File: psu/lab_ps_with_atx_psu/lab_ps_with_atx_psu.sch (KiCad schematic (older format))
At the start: 4 parts, among them CON1 +5V StandBy, U1 LD1117-33

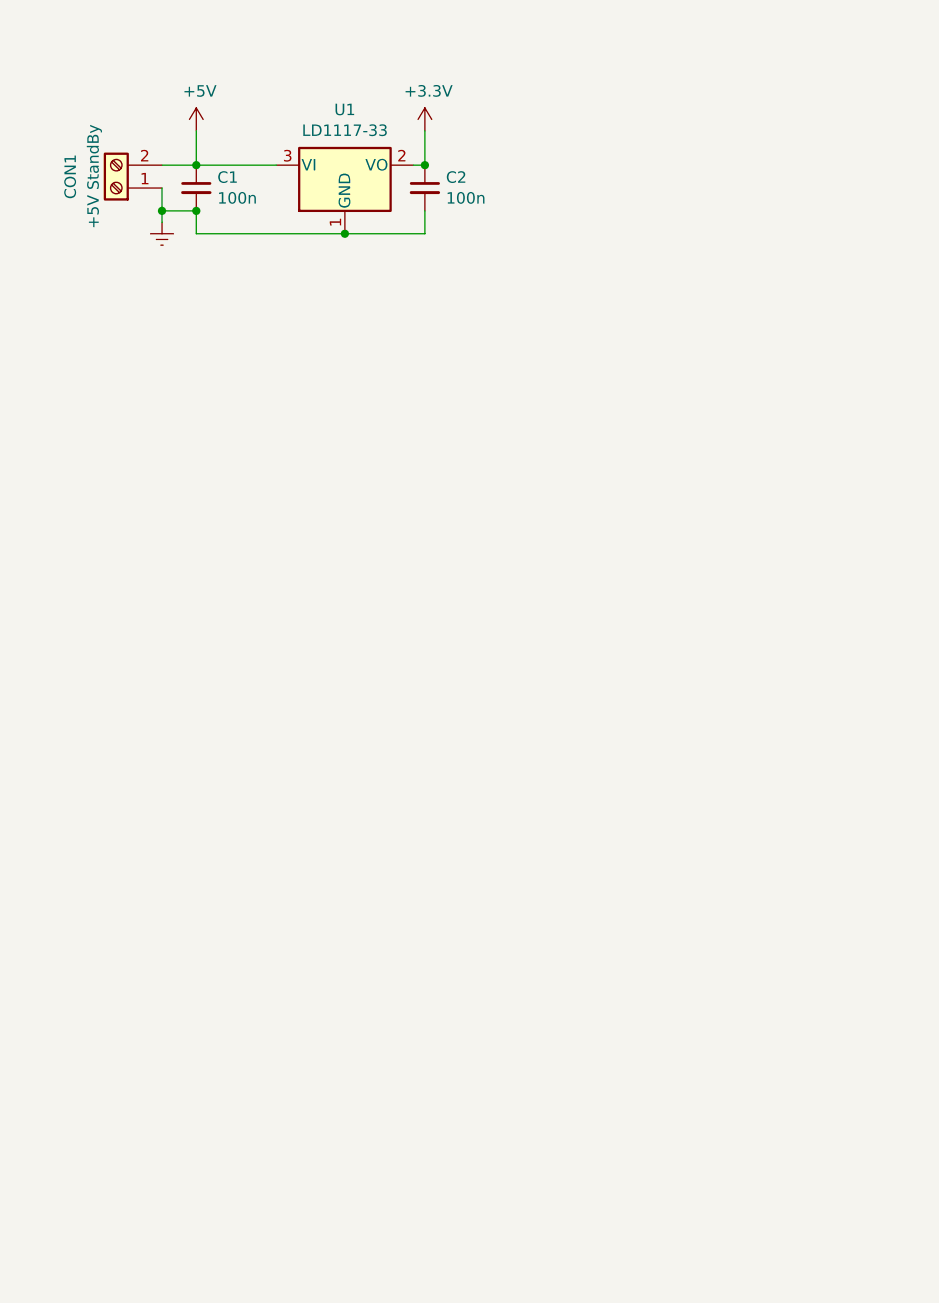
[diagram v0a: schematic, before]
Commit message: microcontroller is added
Please enter the commit message for your changes. Lines starting
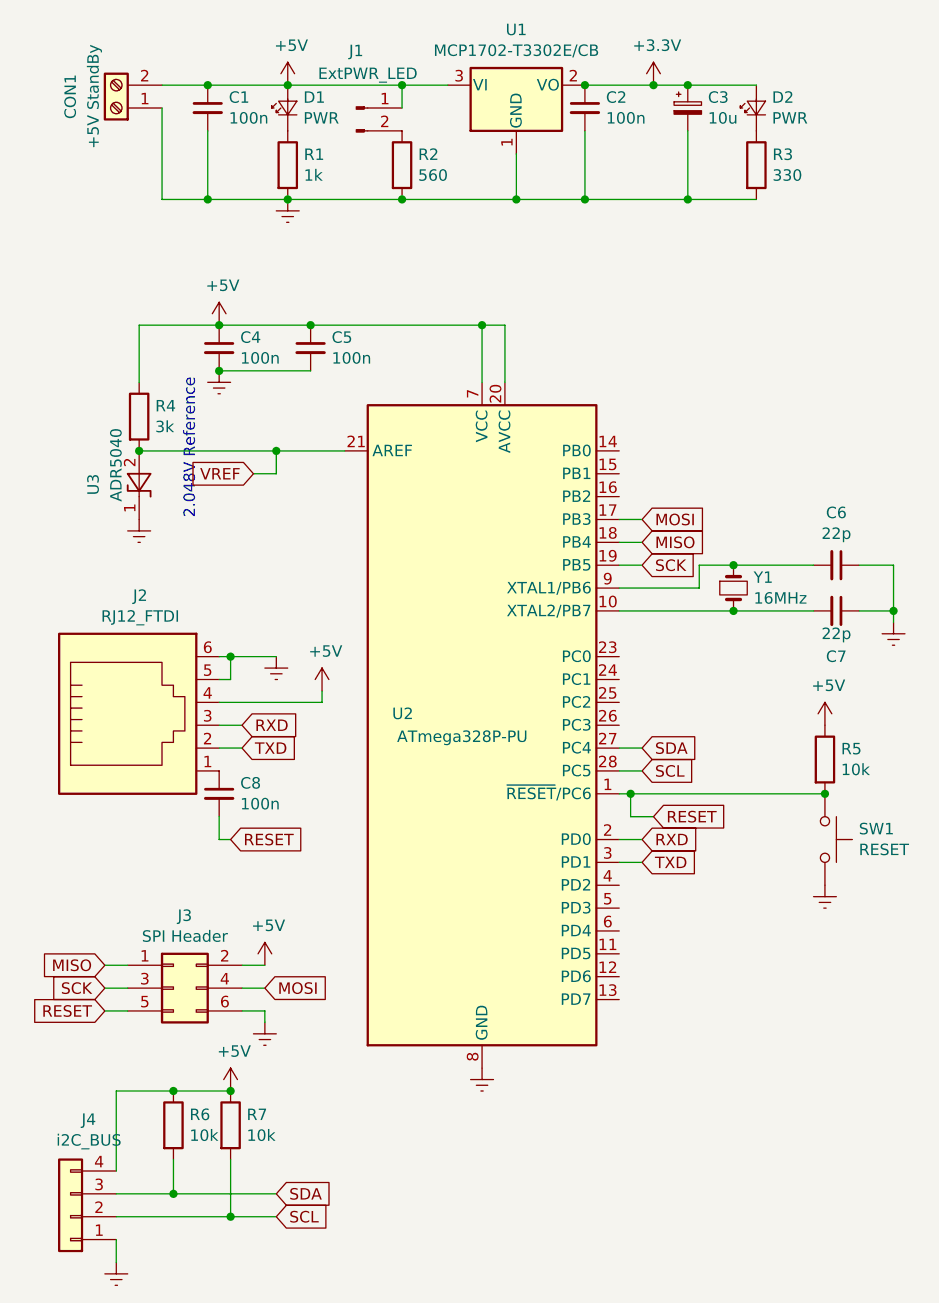
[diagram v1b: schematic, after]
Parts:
- added C3: 10u, Capacitor_SMD:CP_Elec_5x5.3, symbol Device:CP_Small
- added C4, C5, C8: 100n, Capacitor_SMD:C_0805_2012Metric_Pad1.15x1.40mm_HandSolder, symbol Device:C_Small
- added C6, C7: 22p, Capacitor_SMD:C_0805_2012Metric_Pad1.15x1.40mm_HandSolder, symbol Device:C_Small
- added D1, D2: PWR, LED_SMD:LED_0805_2012Metric_Pad1.15x1.40mm_HandSolder, symbol Device:LED_Small
- added J1: ExtPWR_LED, symbol Connector:Conn_01x02_Male
- added J2: RJ12_FTDI, Connector_RJ:RJ12_Amphenol_54601, symbol Connector:RJ12
- added J3: SPI Header, Connector_PinHeader_2.54mm:PinHeader_2x03_P2.54mm_Vertical, symbol Connector_Generic:Conn_02x03_Odd_Even
- added J4: i2C_BUS, Connector_PinHeader_2.54mm:PinHeader_1x04_P2.54mm_Vertical, symbol Connector_Generic:Conn_01x04
- added R1: 1k, Resistor_SMD:R_0805_2012Metric_Pad1.15x1.40mm_HandSolder, symbol Device:R
- added R2: 560, Resistor_SMD:R_0805_2012Metric_Pad1.15x1.40mm_HandSolder, symbol Device:R
- added R3: 330, Resistor_SMD:R_0805_2012Metric_Pad1.15x1.40mm_HandSolder, symbol Device:R
- added R4: 3k, Resistor_SMD:R_0805_2012Metric_Pad1.15x1.40mm_HandSolder, symbol Device:R
- added R5, R6, R7: 10k, Resistor_SMD:R_0805_2012Metric_Pad1.15x1.40mm_HandSolder, symbol Device:R
- added SW1: RESET, Button_Switch_SMD:SW_SPST_EVQPE1, symbol Switch:SW_Push
- added U2: ATmega328P-PU, Package_DIP:DIP-28_W7.62mm, symbol MCU_Microchip_ATmega:ATmega328P-PU
- added U3: ADR5040, Package_TO_SOT_SMD:SOT-23_Handsoldering, symbol Reference_Voltage:LM4040DBZ-10
- added Y1: 16MHz, Crystal:Crystal_SMD_HC49-SD_HandSoldering, symbol Device:Crystal_Small
- C1, C2: footprint Capacitor_THT:C_Disc_D3.0mm_W1.6mm_P2.50mm -> Capacitor_SMD:C_0805_2012Metric_Pad1.15x1.40mm_HandSolder; PN 1002.5992 -> 1000.1122
- U1: value LD1117-33 -> MCP1702-T3302E/CB; footprint Package_TO_SOT_THT:TO-220-3_Vertical -> Package_TO_SOT_SMD:SOT-23_Handsoldering; PN 1002.6083 -> 1003.0653
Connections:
- net +3V3: now also C3.1, D2.2 (A)
- net +5V: now also C4.1, C5.1, D1.2 (A), J1.1 (Pin_1), J2.4, J3.2 (Pin_2), J4.4 (Pin_4), R4.1, R5.1, R6.1, R7.1, U2.20 (AVCC), U2.7 (VCC)
- net Earth: now also C3.2, C4.2, C5.2, C6.1, C7.1, J2.5, J2.6, J3.6 (Pin_6), J4.1 (Pin_1), R1.2, R2.2, R3.2, SW1.2, U2.22 (GND), U2.8 (GND), U3.1 (K)
- new net: C7.2, U2.10 (XTAL2/PB7), Y1.2
- new net: C6.2, U2.9 (XTAL1/PB6), Y1.1
- new net: D1.1 (K), R1.1
- new net: J1.2 (Pin_2), R2.1
- new net: D2.1 (K), R3.1
- new net: C8.1, J2.1
- new net MISO: J3.1 (Pin_1), U2.18 (PB4)
- new net MOSI: J3.4 (Pin_4), U2.17 (PB3)
- new net RESET: C8.2, J3.5 (Pin_5), R5.2, SW1.1, U2.1 (~RESET~/PC6)
- new net RXD: J2.3, U2.2 (PD0)
- new net SCK: J3.3 (Pin_3), U2.19 (PB5)
- new net SCL: J4.2 (Pin_2), R7.2, U2.28 (PC5)
- new net SDA: J4.3 (Pin_3), R6.2, U2.27 (PC4)
- new net TXD: J2.2, U2.3 (PD1)
- new net VREF: R4.2, U2.21 (AREF), U3.2 (A)
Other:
- note added: "2.048V Reference"
- moved on the sheet: CON1, U1
